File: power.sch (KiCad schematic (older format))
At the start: 33 parts, among them J2 4DB-P108-06, J3 39531-1002, J4 39531-1002, J5 Conn_02x03_Counter_Clockwise, U2 i3A, U3 AP7365-33WG-7

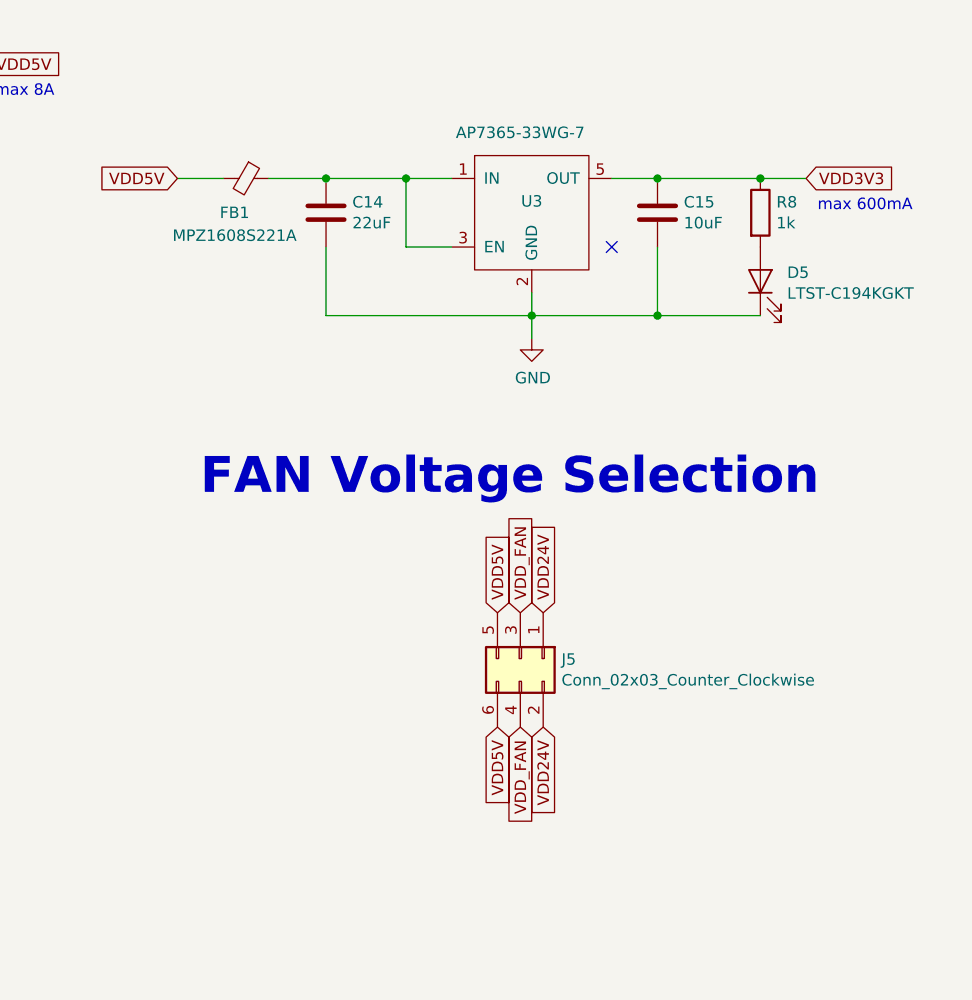
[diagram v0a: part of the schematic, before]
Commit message: Improve Readability
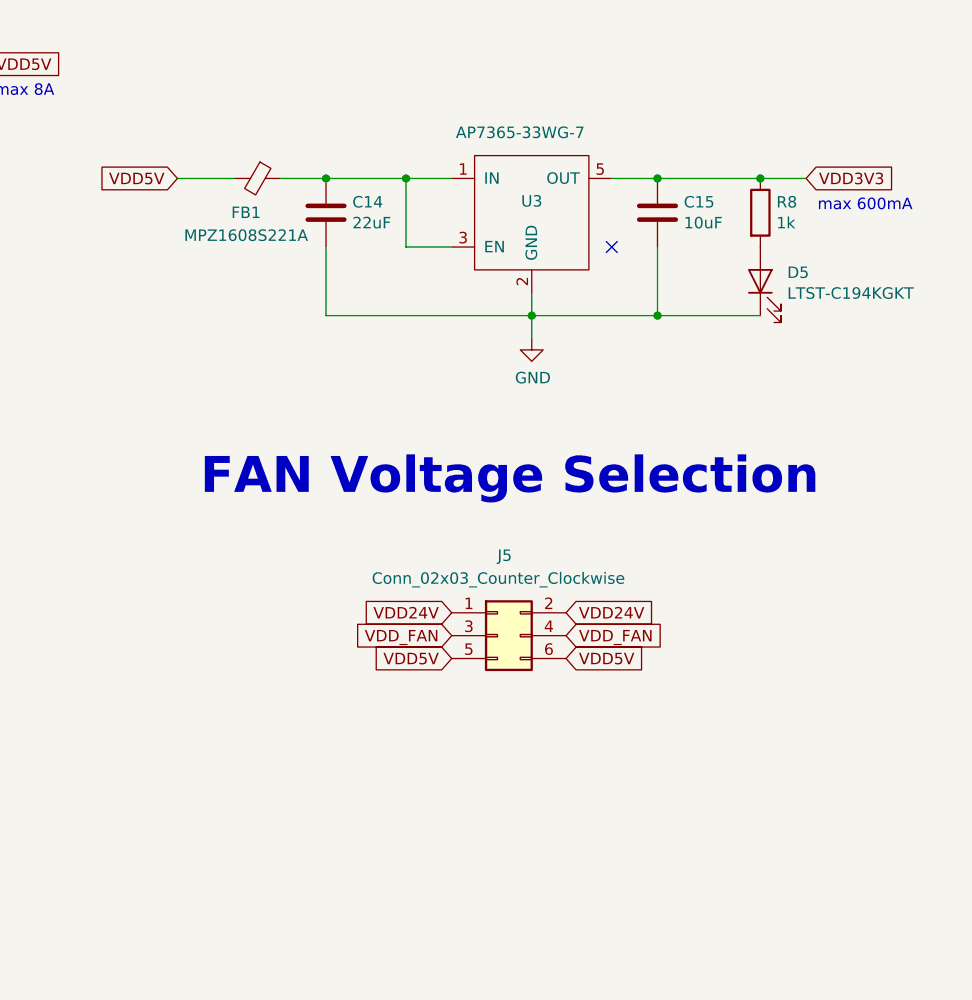
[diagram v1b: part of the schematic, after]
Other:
- moved on the sheet: FB1, J5
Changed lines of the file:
@@
 L Device:Ferrite_Bead_Small FB?
 U 1 1 5BCC4BBE
-P 6650 1750
+P 6700 1750
 AR Path="/5BC1C8A4/5BCC4BBE" Ref="FB?"  Part="1"
 AR Path="/5BC54251/5BCC4BBE" Ref="FB1"  Part="1"
-F 0 "FB1" V 6800 1700 50  0000 C CNN
-F 1 "MPZ1608S221A" V 6900 1700 50  0000 C CNN
-F 2 "Resistor_SMD:R_0603_1608Metric" V 6580 1750 50  0001 C CNN
-F 3 "https://www.mouser.de/datasheet/2/400/eads_commercial_power_mpz1608_en-923650.pdf" H 6650 1750 50  0001 C CNN
-	1    6650 1750
+F 0 "FB1" V 6850 1700 50  0000 C CNN
+F 1 "MPZ1608S221A" V 6950 1700 50  0000 C CNN
+F 2 "Resistor_SMD:R_0603_1608Metric" V 6630 1750 50  0001 C CNN
+F 3 "https://www.mouser.de/datasheet/2/400/eads_commercial_power_mpz1608_en-923650.pdf" H 6700 1750 50  0001 C CNN
+	1    6700 1750
 	0    1    1    0
 $EndComp
 Wire Wire Line
-	6350 1750 6550 1750
+	6350 1750 6600 1750
 $Comp
 L Device:C C15
@@
 Connection ~ 8450 1750
 Wire Wire Line
-	6750 1750 7000 1750
+	6800 1750 7000 1750
 Connection ~ 7000 1750
 Connection ~ 7350 1750
@@
 Text GLabel 1400 5200 2    50   Input ~ 0
 HEAT2_OUT
-Text GLabel 7750 3650 1    50   Input ~ 0
+Text GLabel 7550 3850 0    50   Input ~ 0
 VDD5V
-Text GLabel 7950 3650 1    50   Input ~ 0
+Text GLabel 7550 3650 0    50   Input ~ 0
 VDD24V
-Text GLabel 7850 4150 3    50   Input ~ 0
+Text GLabel 8050 3750 2    50   Input ~ 0
 VDD_FAN
 Text Notes 6450 3150 0    157  ~ 31
@@
 L Connector_Generic:Conn_02x03_Odd_Even J5
 U 1 1 5C045A3C
-P 7850 3850
-F 0 "J5" V 7854 4030 50  0000 L CNN
-F 1 "Conn_02x03_Counter_Clockwise" V 7945 4030 50  0000 L CNN
-F 2 "Connector_PinHeader_2.54mm:PinHeader_2x03_P2.54mm_Vertical" H 7850 3850 50  0001 C CNN
-F 3 "~" H 7850 3850 50  0001 C CNN
-	1    7850 3850
-	0    1    1    0
-$EndComp
-Text GLabel 7850 3650 1    50   Input ~ 0
+P 7750 3750
+F 0 "J5" H 7750 4100 50  0000 L CNN
+F 1 "Conn_02x03_Counter_Clockwise" H 7200 4000 50  0000 L CNN
+F 2 "Connector_PinHeader_2.54mm:PinHeader_2x03_P2.54mm_Vertical" H 7750 3750 50  0001 C CNN
+F 3 "~" H 7750 3750 50  0001 C CNN
+	1    7750 3750
+	1    0    0    -1
+$EndComp
+Text GLabel 7550 3750 0    50   Input ~ 0
 VDD_FAN
-Text GLabel 7750 4150 3    50   Input ~ 0
+Text GLabel 8050 3850 2    50   Input ~ 0
 VDD5V
-Text GLabel 7950 4150 3    50   Input ~ 0
+Text GLabel 8050 3650 2    50   Input ~ 0
 VDD24V
 $EndSCHEMATC
